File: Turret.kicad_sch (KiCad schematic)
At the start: 21 parts, among them J1 Conn_01x04_Pin, J10 Conn_01x04_Pin, J11 Sabre Vertical Header 6, J12 Conn_01x02_Pin, J2 Conn_01x02_Pin, J20 Conn_01x02_Pin, J21 Conn_01x02_Pin, J3 Conn_01x02_Pin, J4 Conn_01x02_Pin, J5 Conn_01x04_Pin, J6 Conn_01x02_Pin, J7 Conn_01x02_Pin, J8 Conn_01x02_Pin, J9 Conn_01x02_Pin

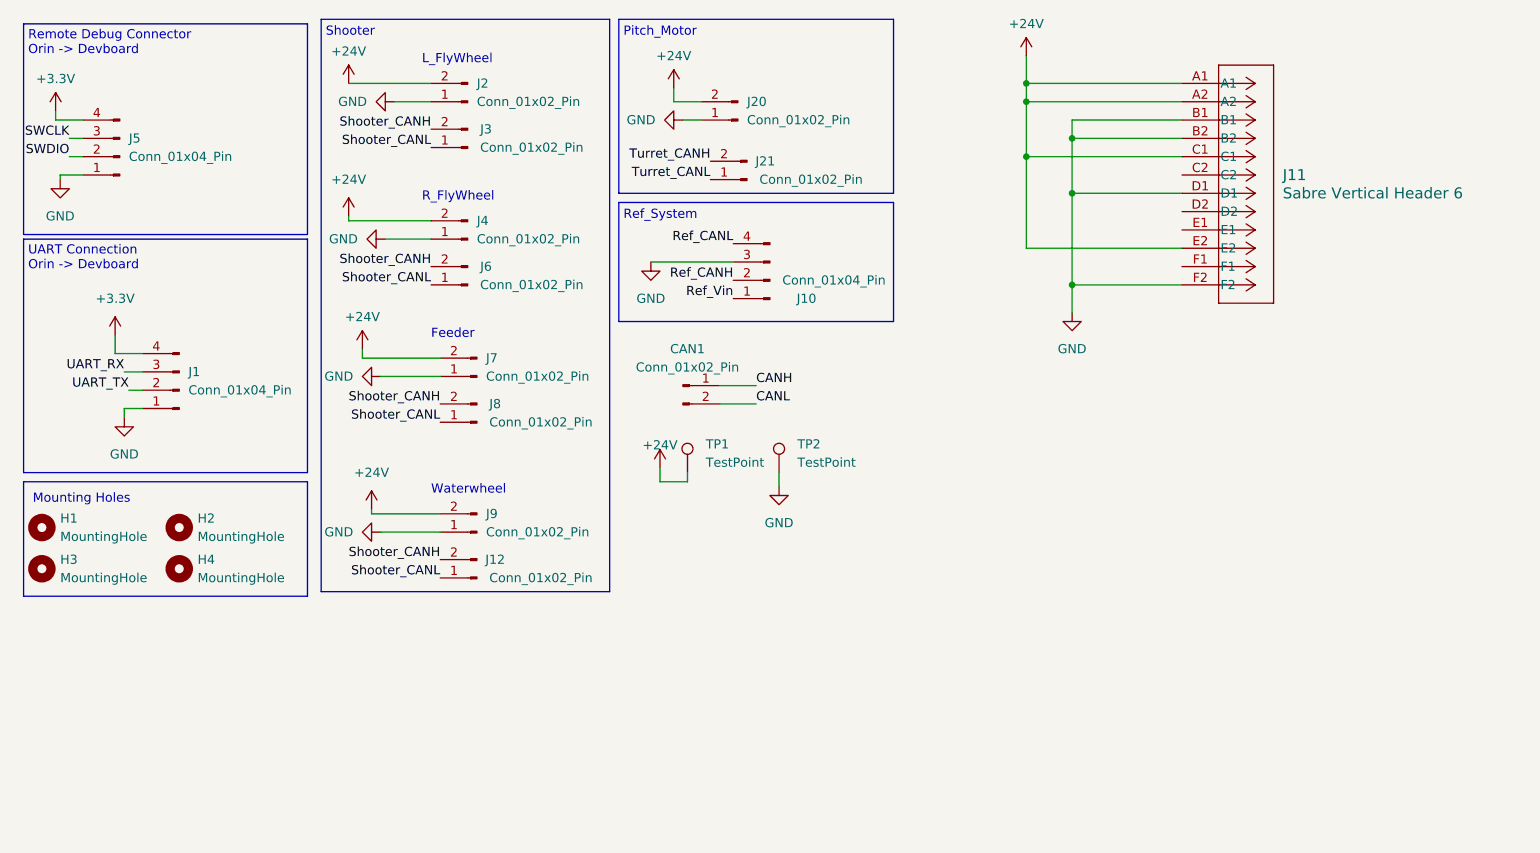
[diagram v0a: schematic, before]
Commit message: Turret change :)
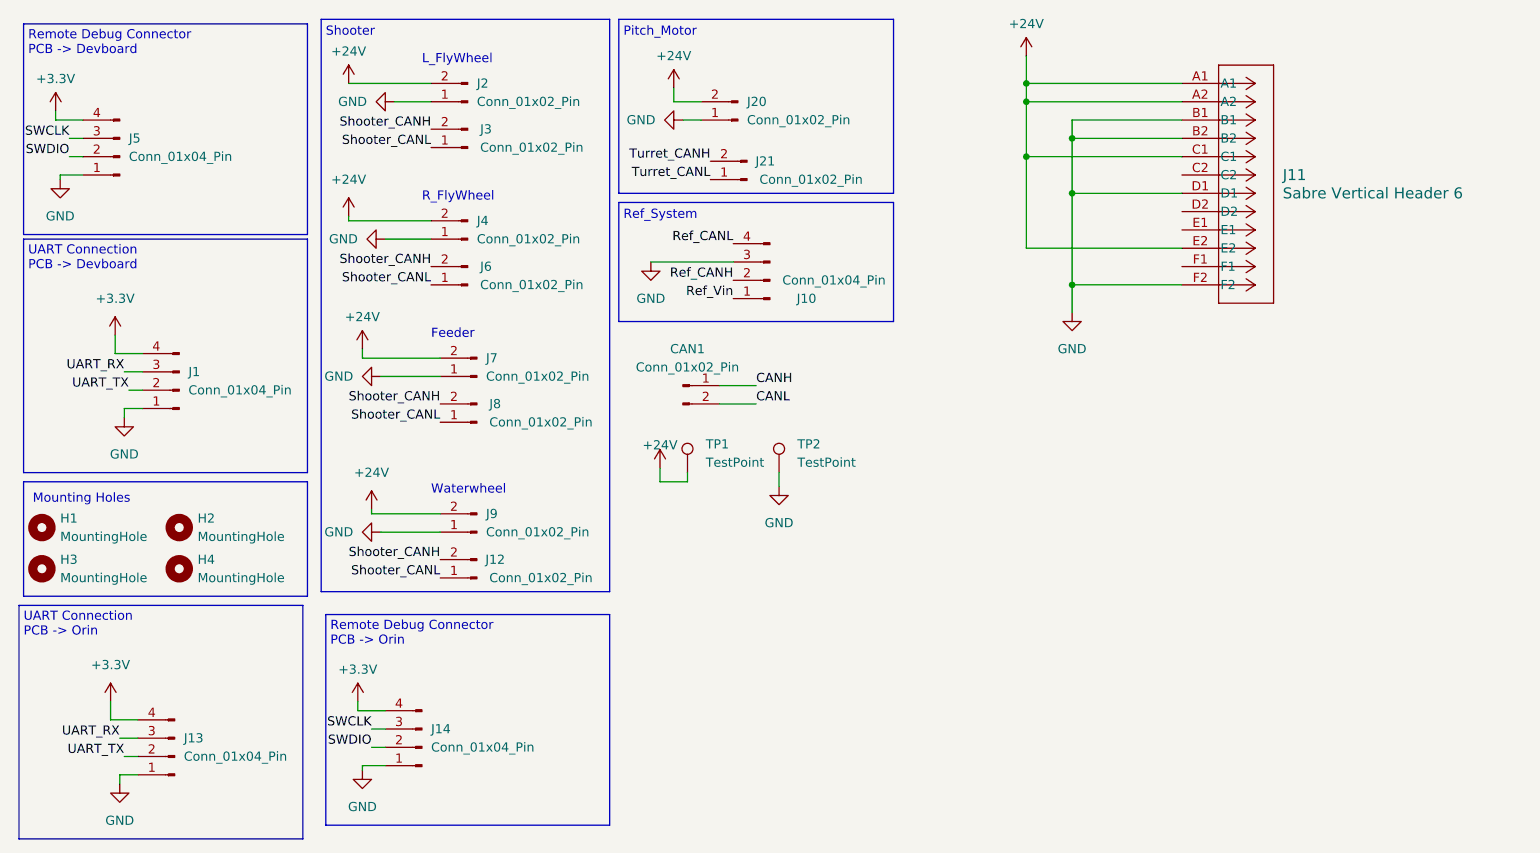
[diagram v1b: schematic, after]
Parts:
- added J13, J14: Conn_01x04_Pin, Connector_JST:JST_GH_BM04B-GHS-TBT_1x04-1MP_P1.25mm_Vertical, symbol Connector:Conn_01x04_Pin
- J1, J5: footprint (none) -> Connector_JST:JST_GH_BM04B-GHS-TBT_1x04-1MP_P1.25mm_Vertical
- J10: footprint Robomasters:866319112100004 -> ICs:866319112100004
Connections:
- net +3.3V: now also J13.4 (Pin_4), J14.4 (Pin_4)
- net GND: now also J13.1 (Pin_1), J14.1 (Pin_1)
- net SWCLK: now also J14.3 (Pin_3)
- net SWDIO: now also J14.2 (Pin_2)
- net UART_RX: now also J13.3 (Pin_3)
- net UART_TX: now also J13.2 (Pin_2)
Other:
- note added: "Remote Debug Connector PCB -> Devboard"
- note added: "Remote Debug Connector PCB -> Orin"
- note added: "UART Connection PCB -> Devboard"
- note added: "UART Connection PCB -> Orin"
- note removed: "Remote Debug Connector Orin -> Devboard"
- note removed: "UART Connection Orin -> Devboard"
